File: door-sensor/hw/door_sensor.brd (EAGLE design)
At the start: 50.5 x 49.5 mm, 10 parts, among them IC1 PRO-MINI

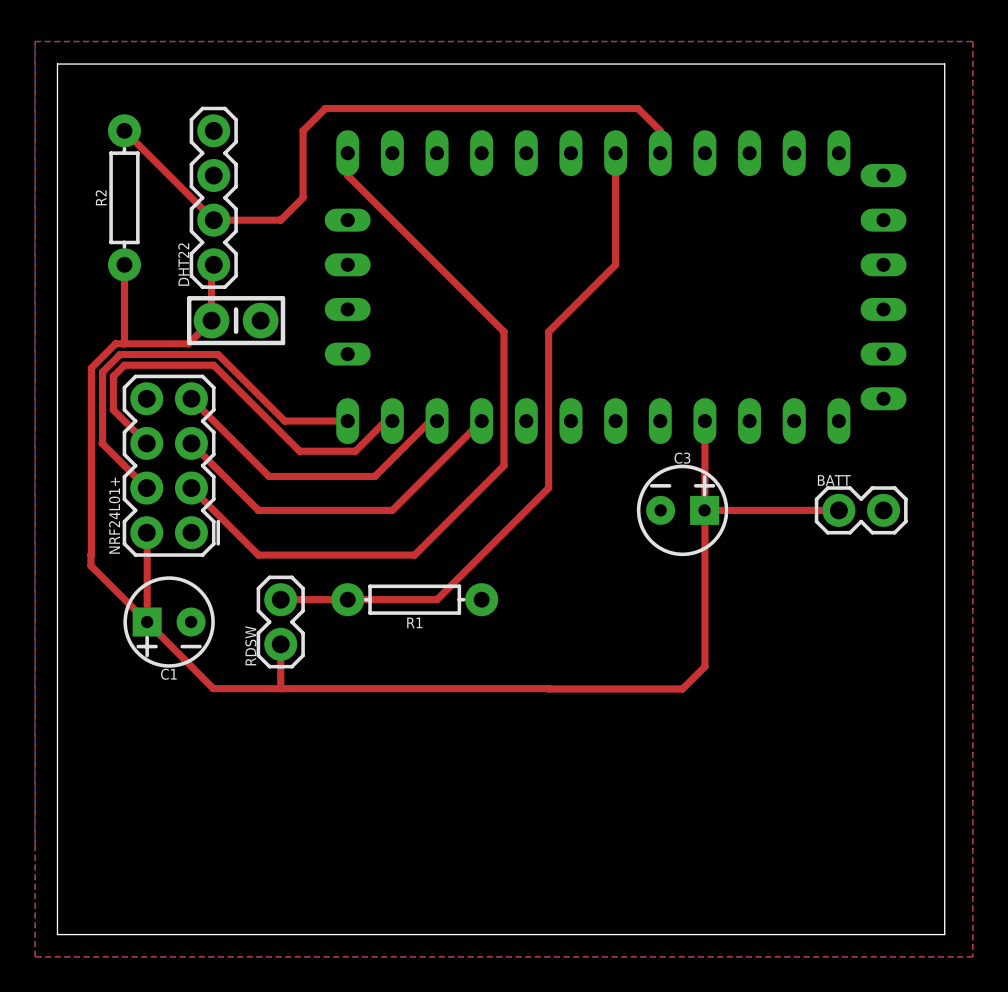
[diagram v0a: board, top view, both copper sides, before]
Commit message: did a load of stuff that I can't remember and hadn't committed for a while
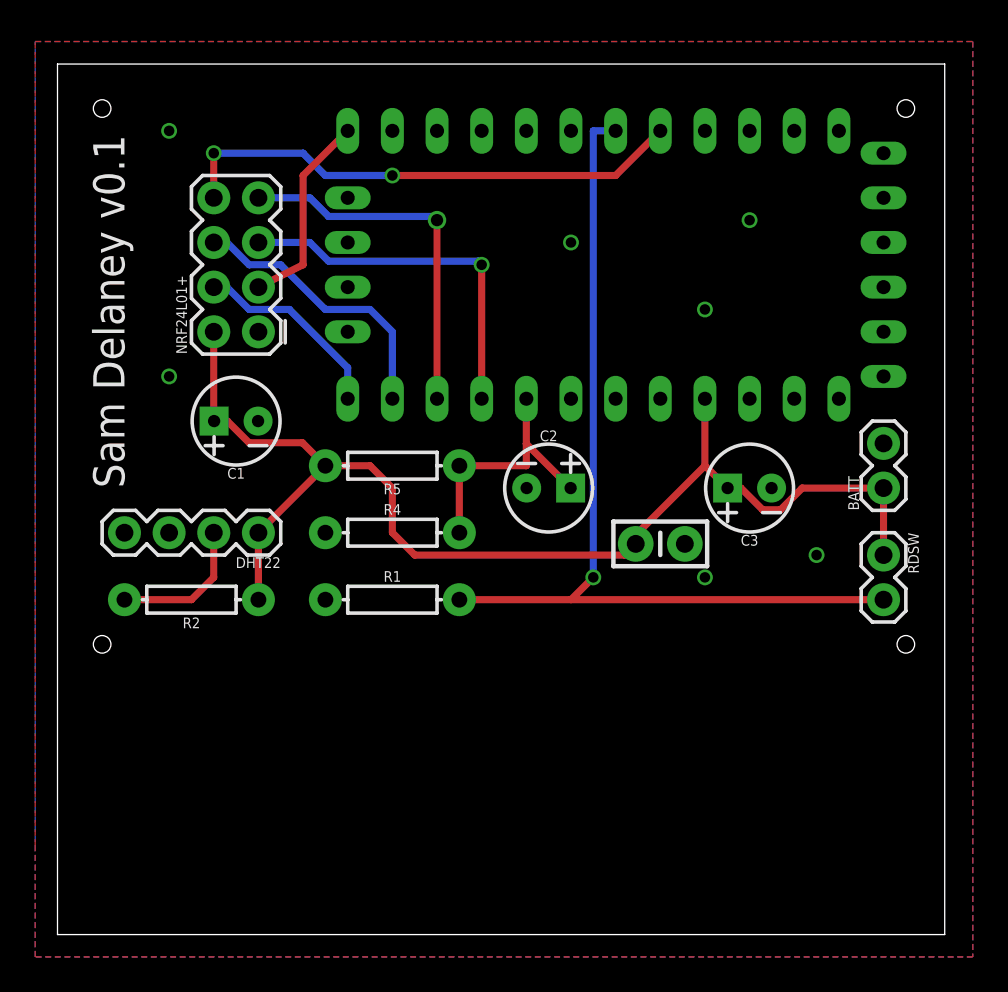
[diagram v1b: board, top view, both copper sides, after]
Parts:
- added C2: 0.47uF, SparkFun-Capacitors:CPOL-RADIAL-2.5MM-5MM
- added R4: 100k, SparkFun-Resistors:AXIAL-0.3
- added R5: 300k, SparkFun-Resistors:AXIAL-0.3
- moved RDSW 34.7 mm to (47.0, 21.6), turned to 270 degrees
- moved C4 27.3 mm to (34.3, 22.2)
- moved R2 23.2 mm to (7.62, 19.1), turned to 180 degrees
- moved DHT22 15.5 mm to (11.4, 22.9), turned to 180 degrees
- moved C1 12.0 mm to (10.2, 29.2)
- moved NRF24L01+ 12.0 mm to (10.2, 38.1)
- moved C3 4.02 mm to (39.4, 25.4), turned to 180 degrees
- moved BATT 2.84 mm to (47.0, 25.4), turned to 90 degrees
- moved R1 1.27 mm to (19.1, 19.1), turned to 0 degrees
- moved IC1 1.27 mm to (17.8, 39.4)
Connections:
- new net BATTO: C2.1, IC1.A0, R4.P$2, R5.P$1
- new net DHT0: IC1.D4
- new net RIRQ: IC1.D2, NRF24L01+.8
- net DHTO: no longer IC1.D2
- net GND: now also C2.2, R4.P$1
- net VCC: now also R5.P$2
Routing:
- net RCE: track 42.9 -> 11.5 mm
- net DHTO: track 39.2 -> 8.15 mm
- net RIRQ: track 0.00 -> 29.5 mm, vias 0 -> 2
- net VCC: track 94.6 -> 68.6 mm
- net BATTO: track 0.00 -> 15.0 mm
- net SWO: track 38.5 -> 52.6 mm, vias 0 -> 1
- net RCS: track 23.6 -> 11.3 mm
- net RMOSI: track 23.5 -> 16.1 mm
- net RMISO: track 17.1 -> 20.8 mm, vias 0 -> 1
- net RSCK: track 20.2 -> 20.8 mm, vias 0 -> 1
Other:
- board text added: "Sam Delaney v0.1"
